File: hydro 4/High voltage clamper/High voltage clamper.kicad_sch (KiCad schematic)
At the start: 7 parts, among them Q1 IRF740

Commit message: Updated clamp board
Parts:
- C1: footprint (none) -> Capacitor_THT:CP_Radial_D8.0mm_P2.50mm
- D2: footprint (none) -> Diode_THT:D_DO-15_P12.70mm_Horizontal
- R1, R2: footprint (none) -> Resistor_THT:R_Axial_DIN0207_L6.3mm_D2.5mm_P7.62mm_Horizontal
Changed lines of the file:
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@@
 			)
 		)
-		(property "Footprint" ""
+		(property "Footprint" "Resistor_THT:R_Axial_DIN0207_L6.3mm_D2.5mm_P7.62mm_Horizontal"
 			(at 138.938 82.55 90)
 			(effects
@@
 			)
 		)
-		(property "Footprint" ""
+		(property "Footprint" "Capacitor_THT:CP_Radial_D8.0mm_P2.50mm"
 			(at 121.6152 87.63 0)
 			(effects
@@
 			)
 		)
-		(property "Footprint" ""
+		(property "Footprint" "Diode_THT:D_DO-15_P12.70mm_Horizontal"
 			(at 113.03 73.66 0)
 			(effects
@@
 			)
 		)
-		(property "Footprint" ""
+		(property "Footprint" "Resistor_THT:R_Axial_DIN0207_L6.3mm_D2.5mm_P7.62mm_Horizontal"
 			(at 102.87 75.438 90)
 			(effects

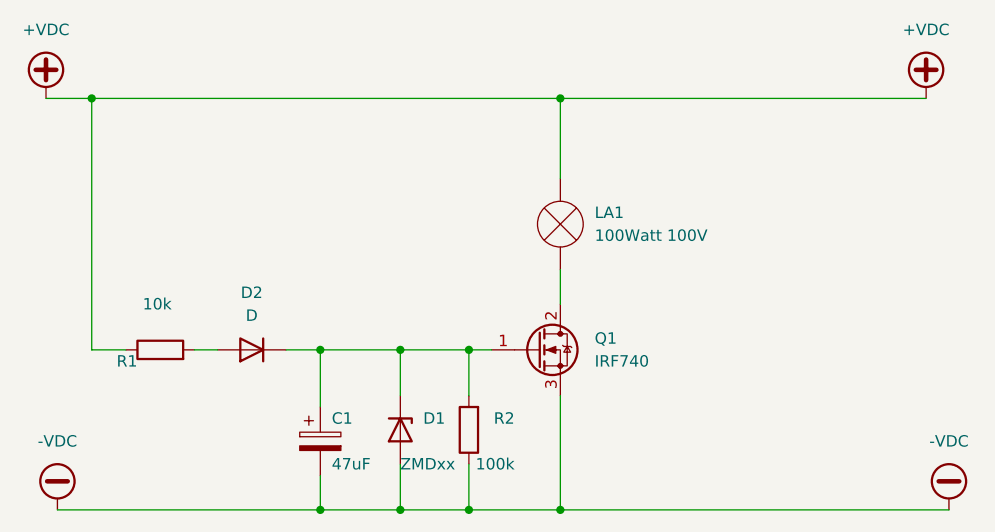
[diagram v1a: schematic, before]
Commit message: Updated schematic
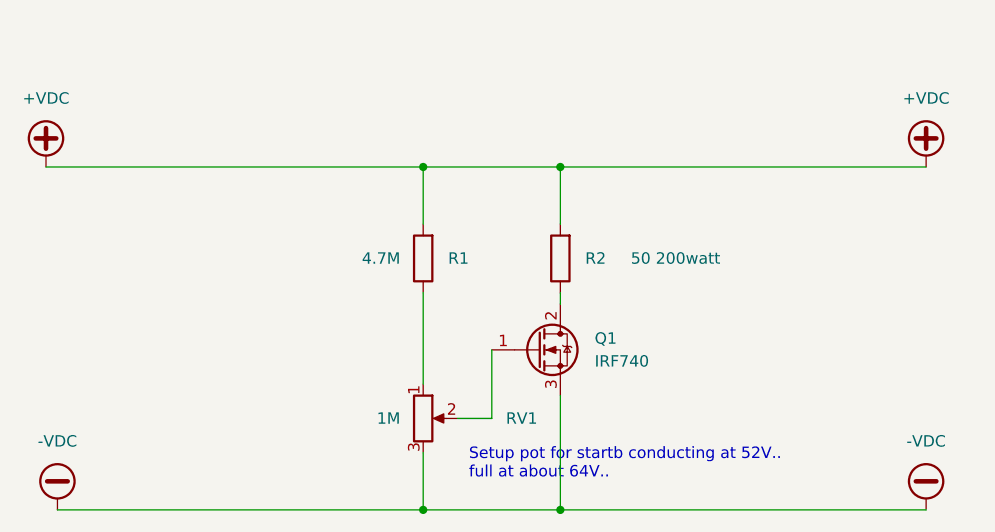
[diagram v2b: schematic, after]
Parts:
- removed C1: 47uF, Capacitor_THT:CP_Radial_D8.0mm_P2.50mm, symbol Device:C_Polarized
- removed D1: ZMDxx, Diode_SMD:D_MiniMELF, symbol Diode:ZMDxx
- removed D2: D, Diode_THT:D_DO-15_P12.70mm_Horizontal, symbol Device:D
- removed LA1: 100Watt 100V, symbol Device:Lamp
- added RV1: 1M, Potentiometer_THT:Potentiometer_ACP_CA14V-15_Vertical_Hole, symbol Device:R_Potentiometer
- R1: value 10k -> 4.7M
- R2: value 100k -> 50 200watt; footprint Resistor_THT:R_Axial_DIN0207_L6.3mm_D2.5mm_P7.62mm_Horizontal -> Resistor_THT:R_Box_L26.0mm_W5.0mm_P20.00mm
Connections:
- net +VDC: now also R1.2, R2.2; no longer R1.1
- net -VDC: now also RV1.3; no longer R2.1
- net at Q1.1 (G): now also RV1.2; no longer R2.2
- net at Q1.2 (D): now also R2.1
- new net: R1.1, RV1.1
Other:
- note added: "Setup pot for startb conducting at 52V.. full at about 64V.."
- moved on the sheet: R1
